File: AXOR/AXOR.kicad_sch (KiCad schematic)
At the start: 44 parts, among them J1 Conn_01x06_Pin, J2 Conn_01x12_Pin, J3 Conn_01x12_Pin, SW1 SW_SPDT, SW2 SW_SPDT, U11 TL074, U13 Aux_flush, U9 LM13700

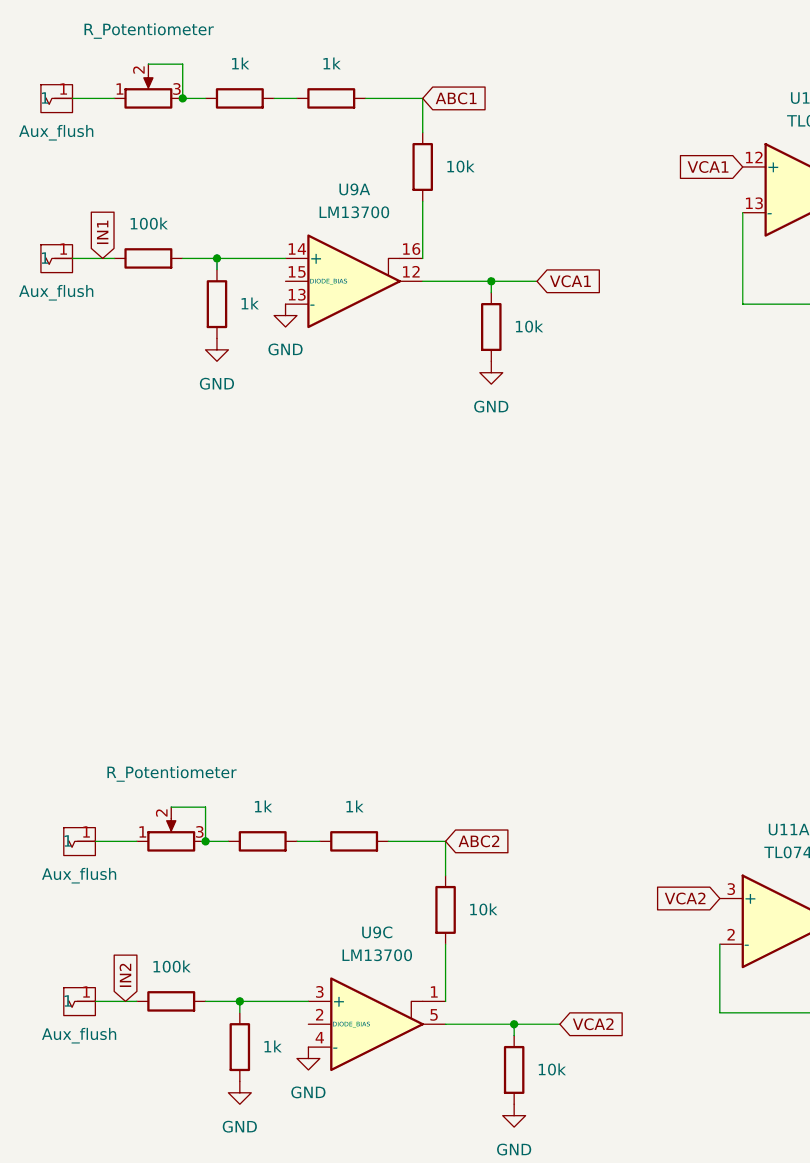
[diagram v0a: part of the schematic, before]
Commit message: Add files via upload
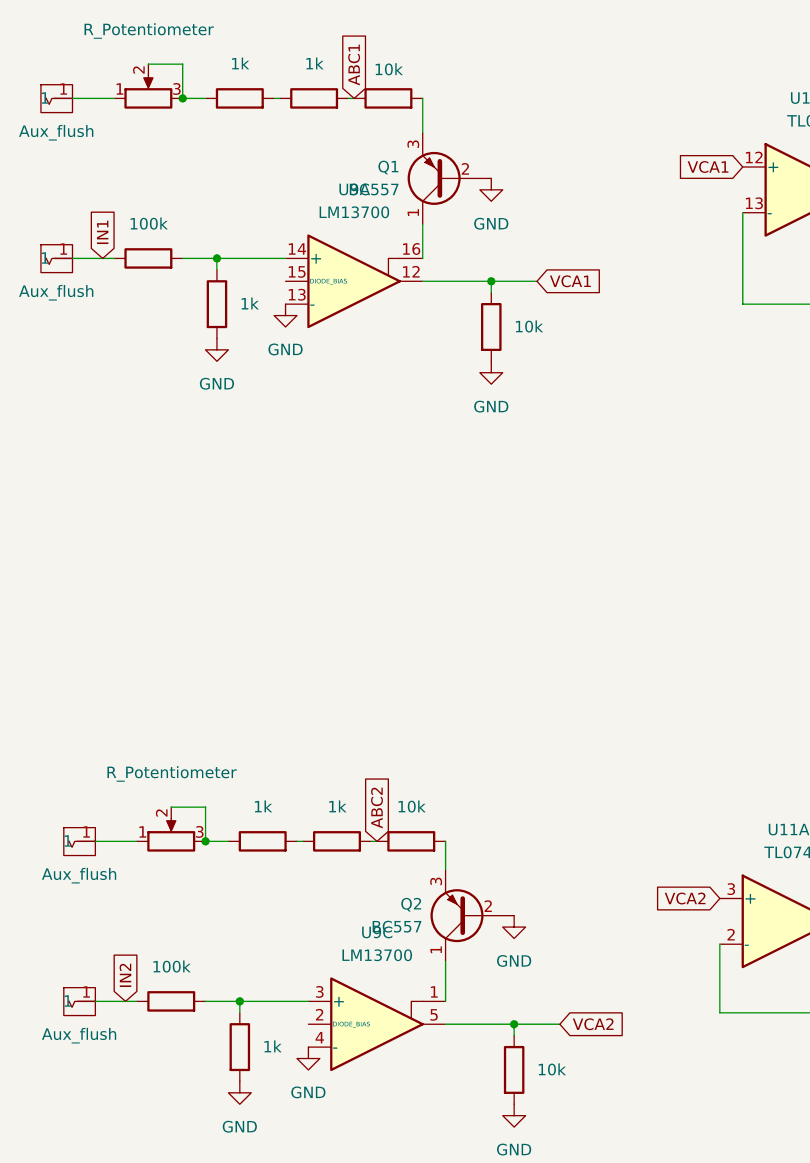
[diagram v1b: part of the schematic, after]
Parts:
- added Q1, Q2: BC557, Package_TO_SOT_THT:TO-92_Inline_Wide, symbol Transistor_BJT:BC557
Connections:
- net GND: now also Q1.2 (B), Q2.2 (B)
- net at U9.16: now also Q1.1 (C); no longer R42.2
- net at R42.2: now also Q2.3 (E); no longer U9.1
- new net: Q1.3 (E), R42.2
- new net: Q2.1 (C), U9.1
